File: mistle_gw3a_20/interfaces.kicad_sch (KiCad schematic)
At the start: 60 parts, among them J11 Joystick 0, J12 Joystick 1, J4 Micro_SD_Card_Det1, J5 HDMI_A, J6 Grove 1125S-4P, J8 EXT UART, SW2 KEY1, SW3 KEY2, U10 74LCX07, U9 74LCX07

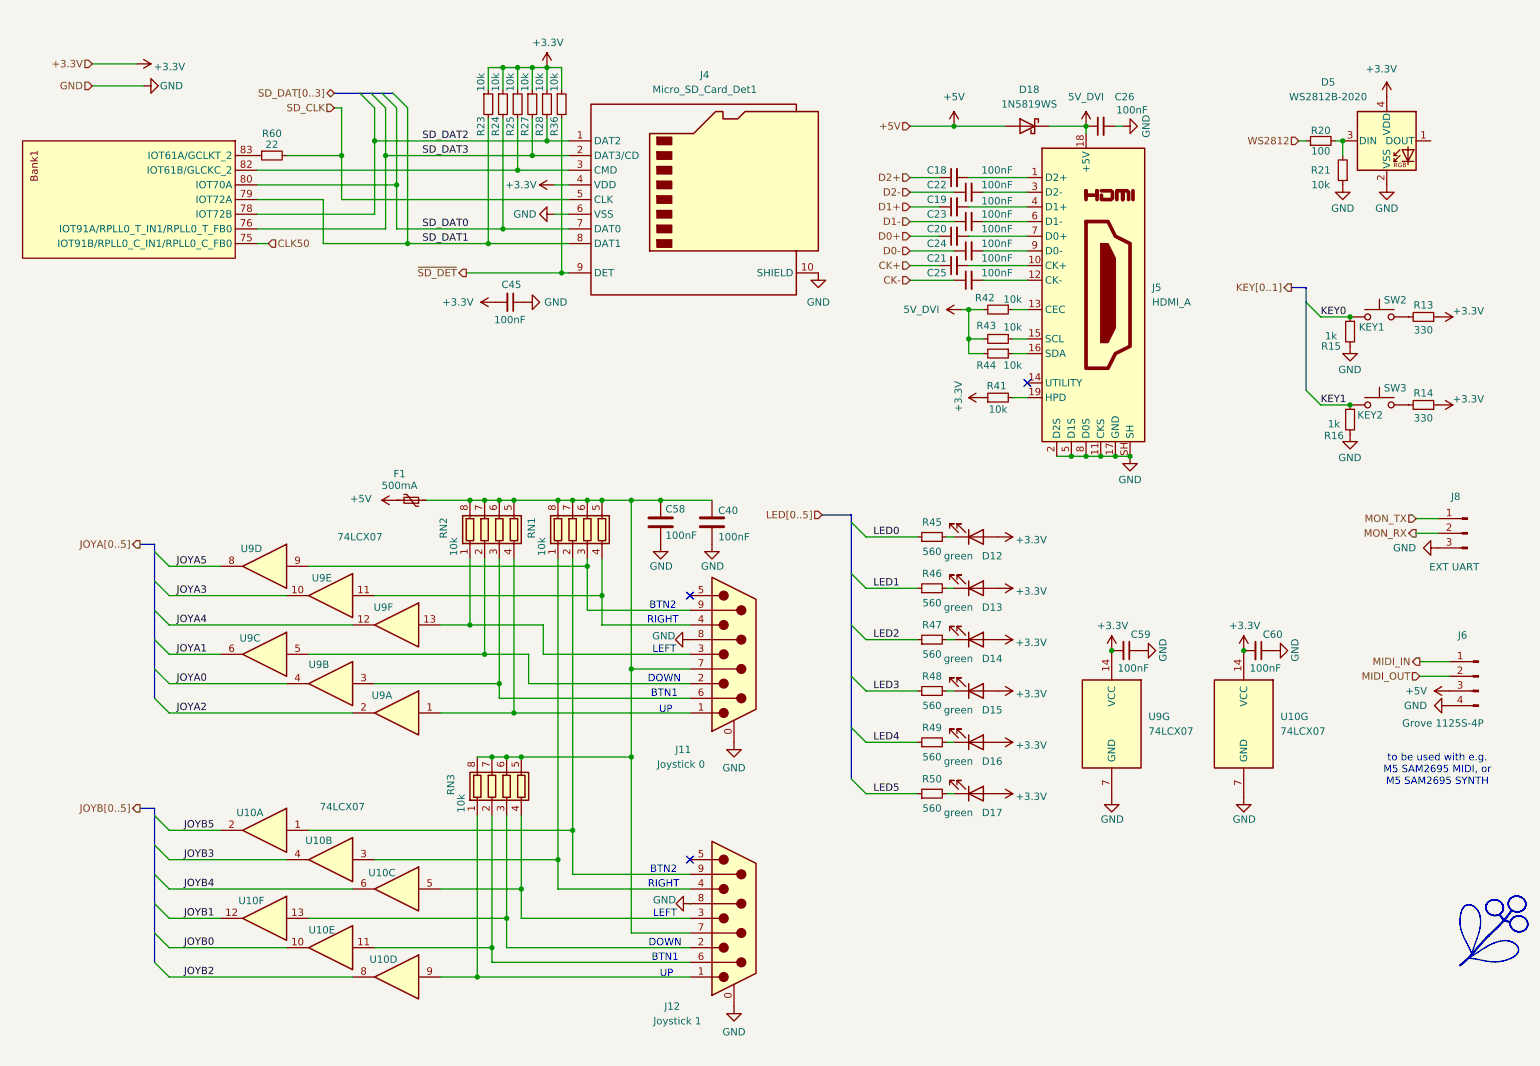
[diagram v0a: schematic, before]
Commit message: Update gw3a dev board
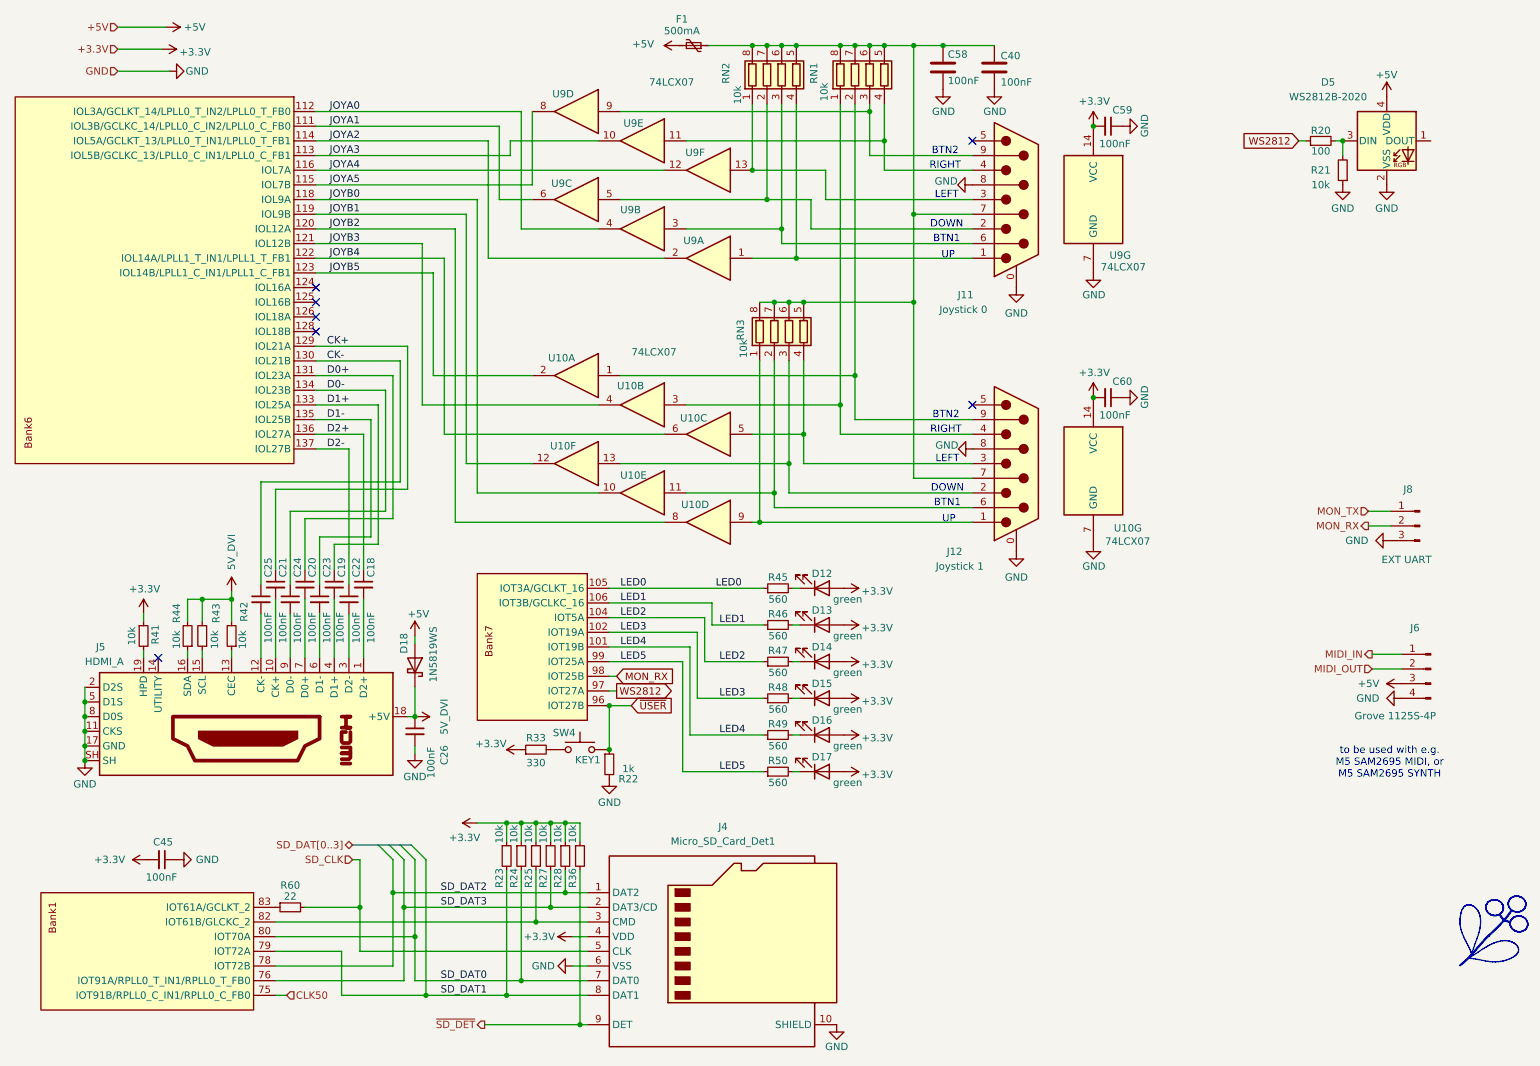
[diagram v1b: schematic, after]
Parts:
- removed R13, R14: 330, Resistor_SMD:R_0402_1005Metric, symbol Device:R_Small
- removed R15, R16: 1k, Resistor_SMD:R_0402_1005Metric, symbol Device:R_Small
- removed SW2: KEY1, Button_Switch_SMD:SW_SPST_TL3342, symbol Switch:SW_Push
- removed SW3: KEY2, Button_Switch_SMD:SW_SPST_TL3342, symbol Switch:SW_Push
- added R22: 1k, Resistor_SMD:R_0402_1005Metric, symbol Device:R_Small
- added R33: 330, Resistor_SMD:R_0402_1005Metric, symbol Device:R_Small
- added SW4: KEY1, Button_Switch_SMD:SW_SPST_TL3342, symbol Switch:SW_Push
- added unit 9 of U7
- added unit 10 of U7
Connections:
- net +3.3V: now also R33.1; no longer D5.4 (VDD)
- net +5V: now also D5.4 (VDD)
- net CK+: now also U7.129 (IOL21A)
- net CK-: now also U7.130 (IOL21B)
- net D0+: now also U7.131 (IOL23A)
- net D0-: now also U7.134 (IOL23B)
- net D1+: now also U7.133 (IOL25A)
- net D1-: now also U7.135 (IOL25B)
- net D2+: now also U7.136 (IOL27A)
- net D2-: now also U7.137 (IOL27B)
- net GND: now also R22.2
- net JOYA0: now also U7.112 (IOL3A/GCLKT_14/LPLL0_T_IN2/LPLL0_T_FB0)
- net JOYA1: now also U7.111 (IOL3B/GCLKC_14/LPLL0_C_IN2/LPLL0_C_FB0)
- net JOYA2: now also U7.114 (IOL5A/GCLKT_13/LPLL0_T_IN1/LPLL0_T_FB1)
- net JOYA3: now also U7.113 (IOL5B/GCLKC_13/LPLL0_C_IN1/LPLL0_C_FB1)
- net JOYA4: now also U7.116 (IOL7A)
- net JOYA5: now also U7.115 (IOL7B)
- net JOYB0: now also U7.118 (IOL9A)
- net JOYB1: now also U7.119 (IOL9B)
- net JOYB2: now also U7.120 (IOL12A)
- net JOYB3: now also U7.121 (IOL12B)
- net JOYB4: now also U7.122 (IOL14A/LPLL1_T_IN1/LPLL1_T_FB1)
- net JOYB5: now also U7.123 (IOL14B/LPLL1_C_IN1/LPLL1_C_FB1)
- net LED0: now also U7.105 (IOT3A/GCLKT_16)
- net LED1: now also U7.106 (IOT3B/GCLKC_16)
- net LED2: now also U7.104 (IOT5A)
- net LED3: now also U7.102 (IOT19A)
- net LED4: now also U7.101 (IOT19B)
- net LED5: now also U7.99 (IOT25A)
- net MON_RX: now also U7.98 (IOT25B)
- net WS2812: now also U7.97 (IOT27A)
- new net: R33.2, SW4.1
- new net ~{USER}: R22.1, SW4.2, U7.96 (IOT27B)
- no-connect marks 3 -> 7
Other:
- moved on the sheet: C18, C19, C20, C21, C22, C23, C24, C25, C26, C40, C45, C58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
